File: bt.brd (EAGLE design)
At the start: 28.9 x 20.3 mm, 16 parts, among them IC1 BLUETOOTH-RN42 HID, Q1 MOSFET-NCHANNELSMD, Q2 MOSFET-NCHANNELSMD

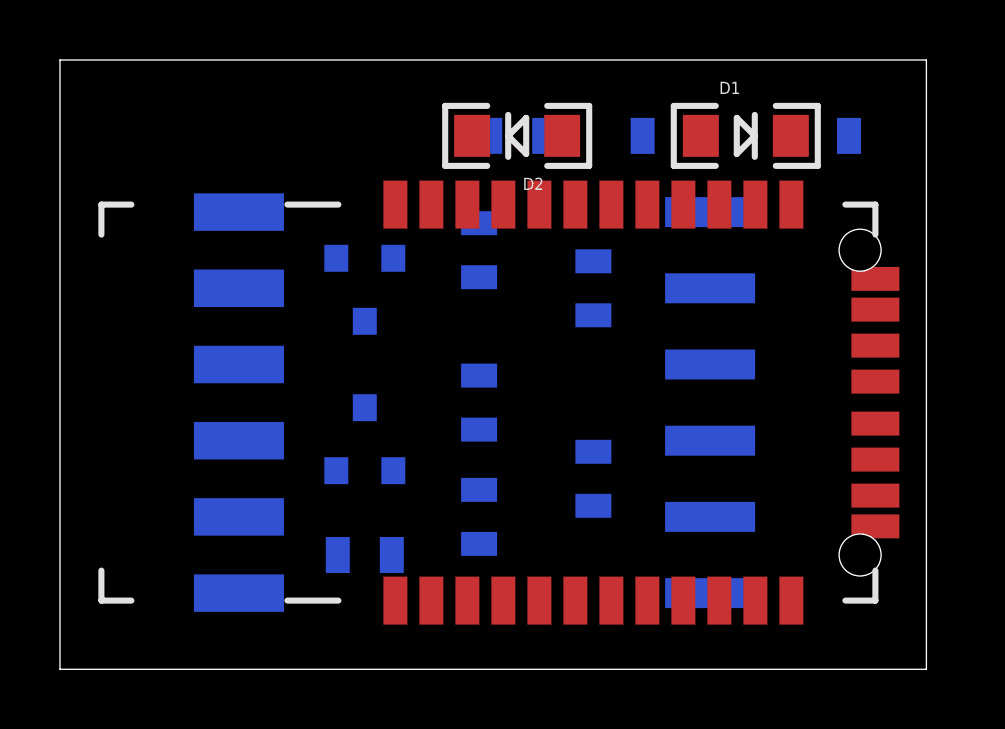
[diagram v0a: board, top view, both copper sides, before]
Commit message: More updates
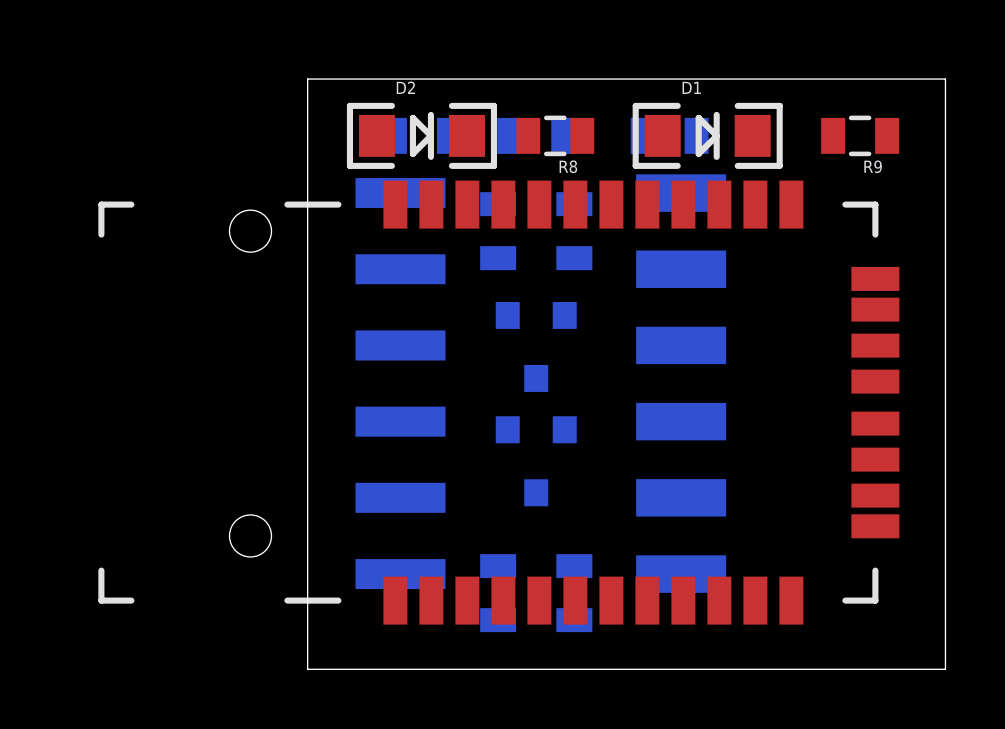
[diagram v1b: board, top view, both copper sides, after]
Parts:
- JP1: value RA 6Pin SMD -> (none); device SparkFun-Connectors:1X06-SMD -> SparkFun-Connectors:1X06-SMD-FEMALE-V2
- JP2: value (none) -> RA 6Pin SMD; device SparkFun-Connectors:1X06-SMD-FEMALE-V2 -> SparkFun-Connectors:1X06-SMD
- moved R2 12.8 mm to (12.1, 17.8), turned to 0 degrees
- moved R3 11.9 mm to (17.1, 2.54)
- moved R5 11.7 mm to (14.6, 14.6), turned to 270 degrees
- moved R6 10.0 mm to (17.1, 14.6)
- moved Q1 8.08 mm to (15.9, 6.99)
- moved Q2 6.54 mm to (15.9, 10.8), turned to 180 degrees
- moved R4 6.38 mm to (14.6, 2.54)
- moved R1 5.43 mm to (15.9, 17.8), turned to 0 degrees
- moved R7 5.08 mm to (20.3, 17.8), turned to 180 degrees
- moved JP2 3.86 mm to (6.35, 9.53)
- moved R8 3.81 mm to (16.5, 17.8), flipped to the top, turned to 180 degrees
- moved D2 3.18 mm to (12.1, 17.8), turned to 0 degrees
- moved JP1 2.62 mm to (24.1, 9.53)
- moved R9 1.27 mm to (26.7, 17.8), flipped to the top
- moved D1 1.27 mm to (21.6, 17.8)
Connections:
- removed net N$2: JP2.2
- net 3.3V: now also JP1.6; no longer JP2.6
- net UART_CTS_5V: now also JP2.5; no longer JP1.5
- net UART_RTS_5V: now also JP2.2; no longer JP1.2
- net UART_RX_5V: now also JP2.3; no longer JP1.3
- net UART_TX_5V: now also JP2.4; no longer JP1.4
- net USB_D+: now also JP1.4; no longer JP2.4
- net USB_D-: now also JP1.3; no longer JP2.3
- net VCC: now also JP1.5, JP2.6; no longer JP1.6, JP2.5
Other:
- board size 28.9 x 20.3 mm -> 21.3 x 19.7 mm
- board text added: "3.3V"
- board text added: "CTS"
- board text added: "D+"
- board text added: "D-"
- board text added: "GND"
- board text added: "NC"
- board text added: "RTS"
- board text added: "RX"
- board text added: "TX"
- board text added: "VCC"
